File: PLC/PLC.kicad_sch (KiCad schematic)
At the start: 88 parts, among them J1 HR911105A_C12074, J2 HR911105A_C12074, U1 STM32H743ZIT6, U10 MELF-MFR02041/4WS49.9KΩFT50, U11 MELF-MFR02041/4WS49.9KΩFT50, U12 TPS23881RTQR, U2 M24C16-RMN6TP, U3 LAN9252I/ML, U4 MELF-MFR02041/4WS49.9KΩFT50, U5 MELF-MFR02041/4WS49.9KΩFT50, U6 MELF-MFR02041/4WS49.9KΩFT50, U7 MELF-MFR02041/4WS49.9KΩFT50, U8 MELF-MFR02041/4WS49.9KΩFT50, U9 MELF-MFR02041/4WS49.9KΩFT50, X2 X322512MSB4SI, X3 X322525MSB4SI

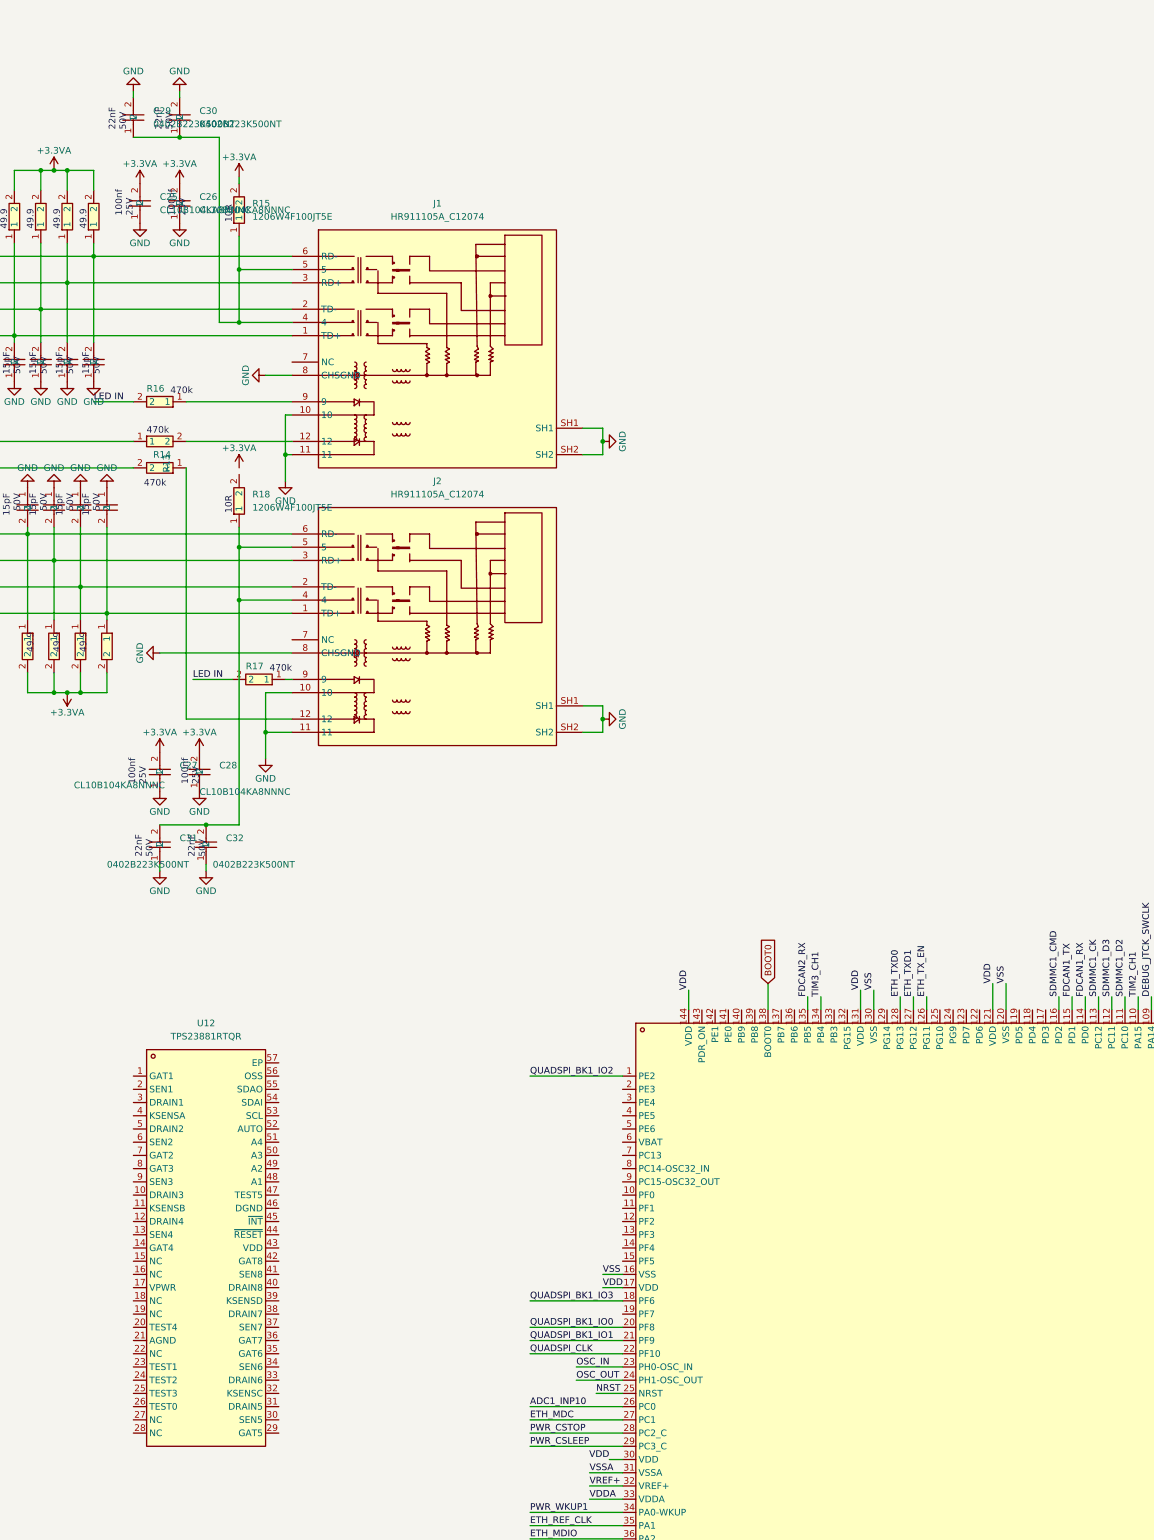
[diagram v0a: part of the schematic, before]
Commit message: Add files via upload
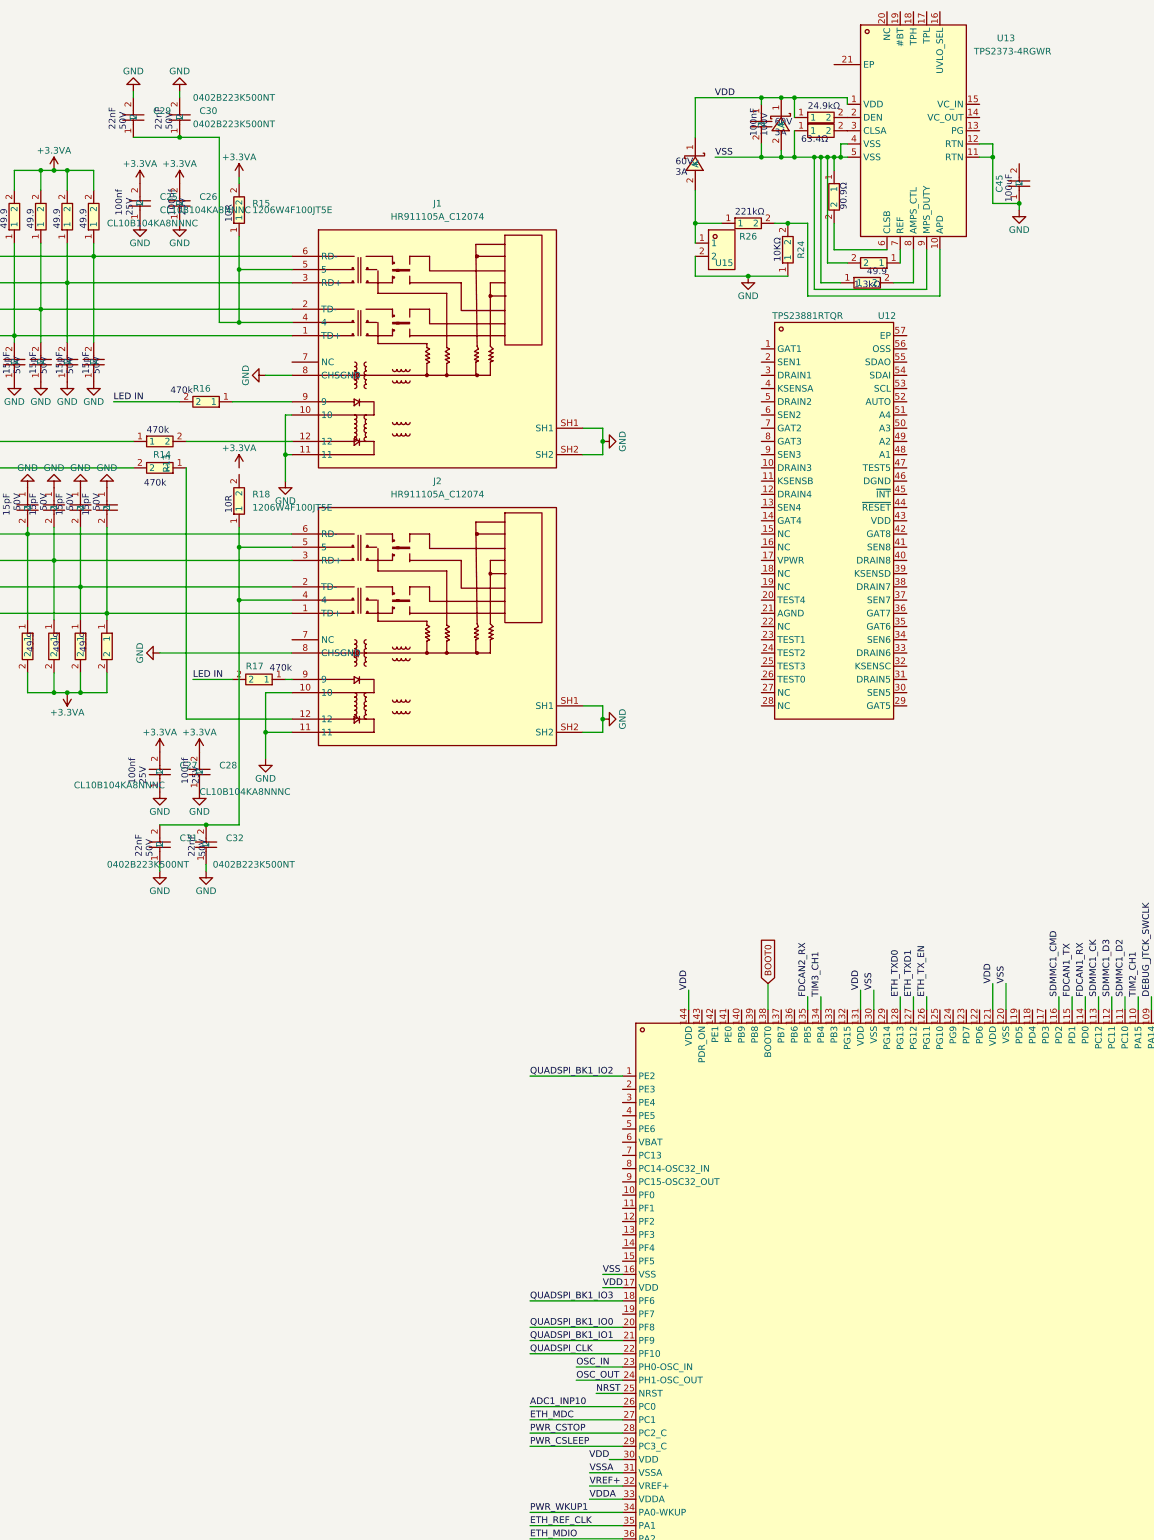
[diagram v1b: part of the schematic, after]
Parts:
- added C45: CL31A107MQHNNNE, easyeda2kicad:C1206, symbol easyeda2kicad:CL31A107MQHNNNE
- added C47: CL21B104KCFNNNE, easyeda2kicad:C0805, symbol easyeda2kicad:CL21B104KCFNNNE
- added D1, D2: SS36, easyeda2kicad:SMA_L4.3-W2.6-LS5.2-RD, symbol easyeda2kicad:SS36
- added R20: 0805W8F2492T5E, easyeda2kicad:R0805, symbol easyeda2kicad:0805W8F2492T5E
- added R22: RC-02W90R9FT, easyeda2kicad:R0402, symbol easyeda2kicad:RC-02W90R9FT
- added R23: ERJ3EKF63R4V, easyeda2kicad:R0603, symbol easyeda2kicad:ERJ3EKF63R4V
- added R24: 0805W8F1002T5E, easyeda2kicad:R0805, symbol easyeda2kicad:0805W8F1002T5E
- added R25: 0805W8F1301T5E, easyeda2kicad:R0805, symbol easyeda2kicad:0805W8F1301T5E
- added R26: 1206W4F2213T5E, easyeda2kicad:R1206, symbol easyeda2kicad:1206W4F2213T5E
- added U13: TPS2373-4RGWR, easyeda2kicad:VQFN-20_L5.0-W5.0-P0.65-BL-EP2.2, symbol easyeda2kicad:TPS2373-4RGWR
- added U14: MELF-MFR02041/4WS49.9KΩFT50, easyeda2kicad:RES-SMD_L3.5-W1.5, symbol easyeda2kicad:MELF-MFR02041_4WS49.9KΩFT50
- added U15: KF301-5.0-2P, easyeda2kicad:CONN-TH_P5.00_KF301-5.0-2P, symbol easyeda2kicad:KF301-5.0-2P
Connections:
- net +3.3V: now also C47.1, D1.1 (K), D2.1 (K), R20.1, U13.1 (VDD)
- net GND: now also C45.1, C47.2, D2.2 (A), R22.1, R23.1, R24.1, R25.1, U13.11 (RTN), U13.12 (RTN), U13.4 (VSS), U13.5 (VSS), U13.9 (MPS_DUTY), U14.2, U15.2
- new net: R20.2, U13.2 (DEN)
- new net: R24.2, R26.2, U13.10 (APD)
- new net: D1.2 (A), R26.1, U15.1
- new net: R23.2, U13.3 (CLSA)
- new net: U13.7 (REF), U14.1
- new net: R22.2, U13.6 (CLSB)
- new net: R25.2, U13.8 (AMPS_CTL)
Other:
- note added: "1.3kΩ"
- note added: "100nF 100V"
- note added: "100uF"
- note added: "10KΩ"
- note added: "221kΩ"
- note added: "24.9kΩ"
- note added: "60V 3A"
- note added: "63.4Ω"
- note added: "90.9Ω"
- moved on the sheet: R16, U12
